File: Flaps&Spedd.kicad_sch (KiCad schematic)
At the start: 19 parts, among them J1 CAN-In, J2 CAN-Out, U1 SN65HVD230

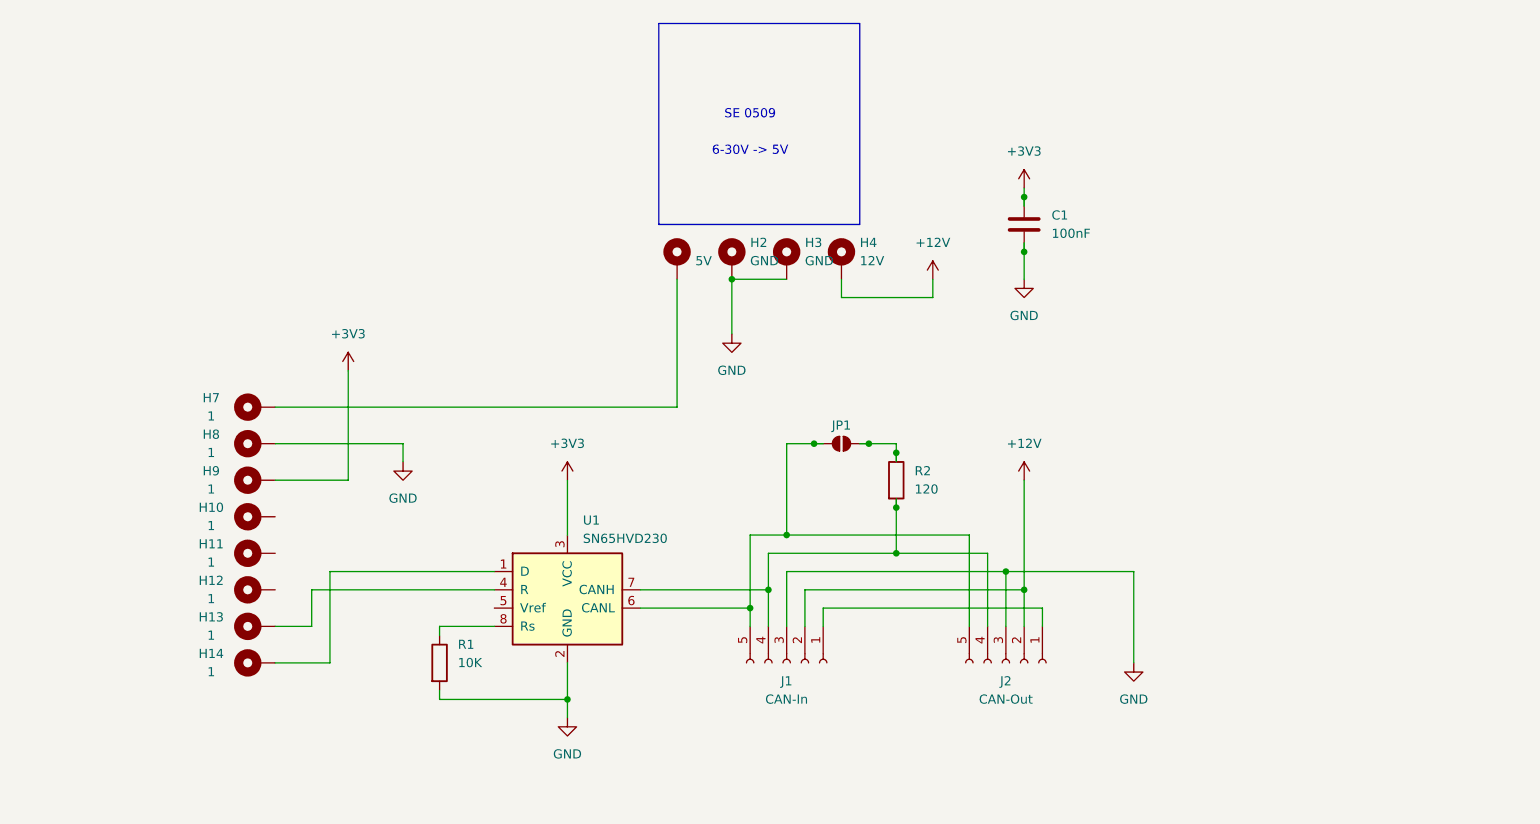
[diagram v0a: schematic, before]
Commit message: v3
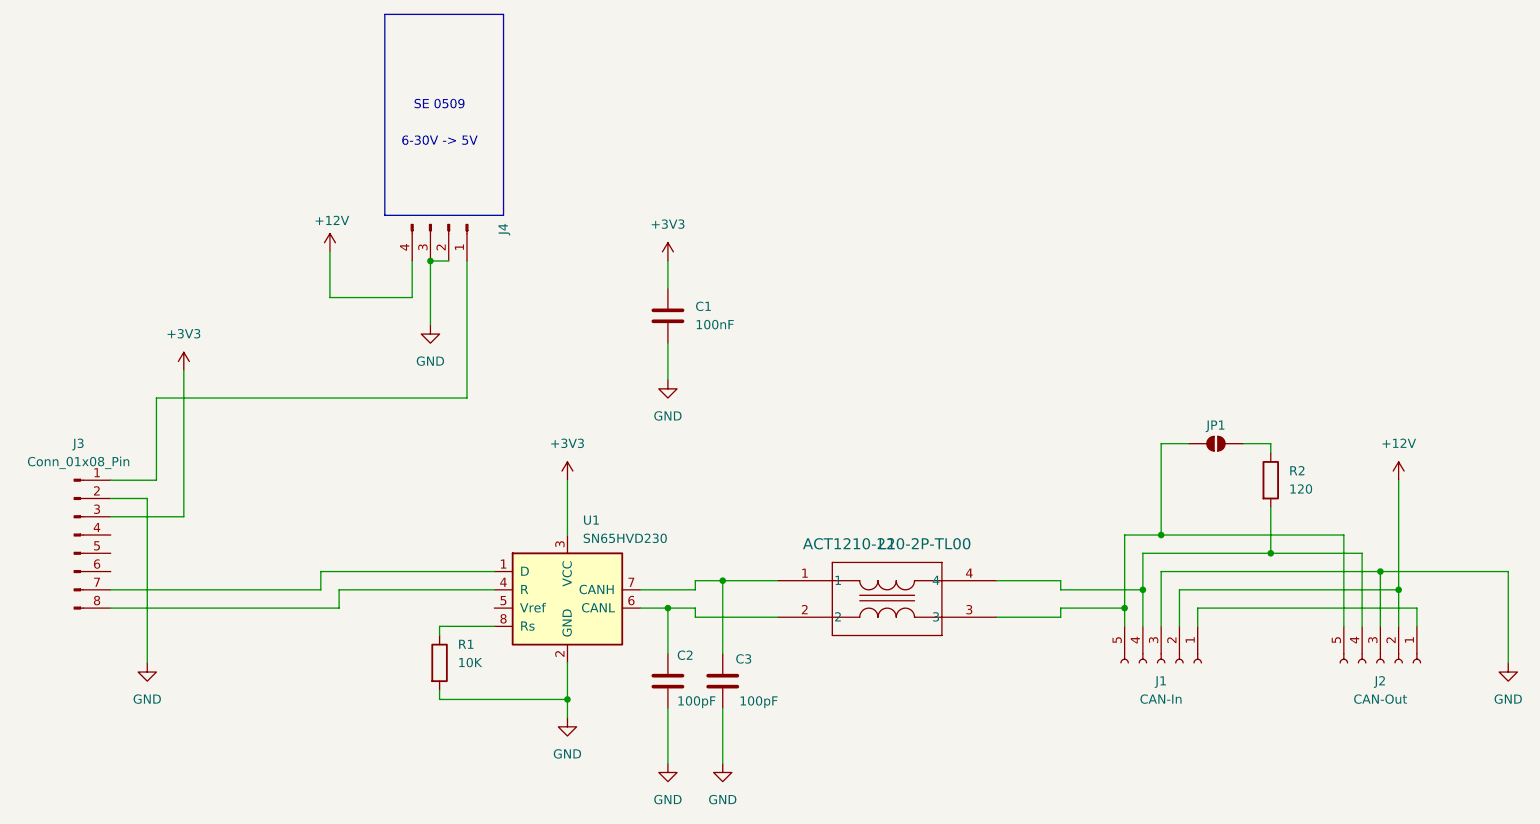
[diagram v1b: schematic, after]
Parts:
- removed H1: 5V, Connector_PinHeader_1.27mm:PinHeader_1x01_P1.27mm_Vertical, symbol Mechanical:MountingHole_Pad
- removed H10, H11, H12, H13, H14, H7, H8, H9: 1, Connector_PinHeader_1.27mm:PinHeader_1x01_P1.27mm_Vertical, symbol Mechanical:MountingHole_Pad
- removed H2, H3: GND, Connector_PinHeader_1.27mm:PinHeader_1x01_P1.27mm_Vertical, symbol Mechanical:MountingHole_Pad
- removed H4: 12V, Connector_PinHeader_1.27mm:PinHeader_1x01_P1.27mm_Vertical, symbol Mechanical:MountingHole_Pad
- added C2, C3: 100pF, Resistor_SMD:R_1206_3216Metric_Pad1.30x1.75mm_HandSolder, symbol Device:C
- added J3: Conn_01x08_Pin, Connector_PinSocket_2.54mm:PinSocket_1x08_P2.54mm_Vertical, symbol Connector:Conn_01x08_Pin
- added J4: Conn_01x04_Pin, Connector_PinSocket_2.54mm:PinSocket_1x04_P2.54mm_Vertical, symbol Connector:Conn_01x04_Pin
- added L1: ACT1210-220-2P-TL00, ACT1210_TDK, symbol Mechanical:ACT1210-220-2P-TL00
- C1: footprint Capacitor_SMD:C_0201_0603Metric -> Resistor_SMD:R_1206_3216Metric_Pad1.30x1.75mm_HandSolder
- R1, R2: footprint Resistor_SMD:R_0201_0603Metric -> Resistor_SMD:R_1206_3216Metric_Pad1.30x1.75mm_HandSolder
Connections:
- net +12V: now also J4.4 (Pin_4)
- net +3V3: now also J3.3 (Pin_3)
- net GND: now also C2.2, C3.2, J3.2 (Pin_2), J4.2 (Pin_2), J4.3 (Pin_3)
- net at U1.1 (D): now also J3.7 (Pin_7)
- net at J1.4 (Pin_4), J2.4 (Pin_4), R2.2: now also L1.4; no longer U1.7 (CANH)
- net at J1.5 (Pin_5), J2.5 (Pin_5), JP1.1 (A): now also L1.3; no longer U1.6 (CANL)
- net at U1.4 (R): now also J3.8 (Pin_8)
- new net: C3.1, L1.1, U1.7 (CANH)
- new net: J3.1 (Pin_1), J4.1 (Pin_1)
- new net: C2.1, L1.2, U1.6 (CANL)
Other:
- moved on the sheet: C1, J1, J2, JP1, R2
